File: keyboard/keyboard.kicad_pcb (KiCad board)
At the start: 2 copper layers, 127.1 x 77.5 mm, 21 parts

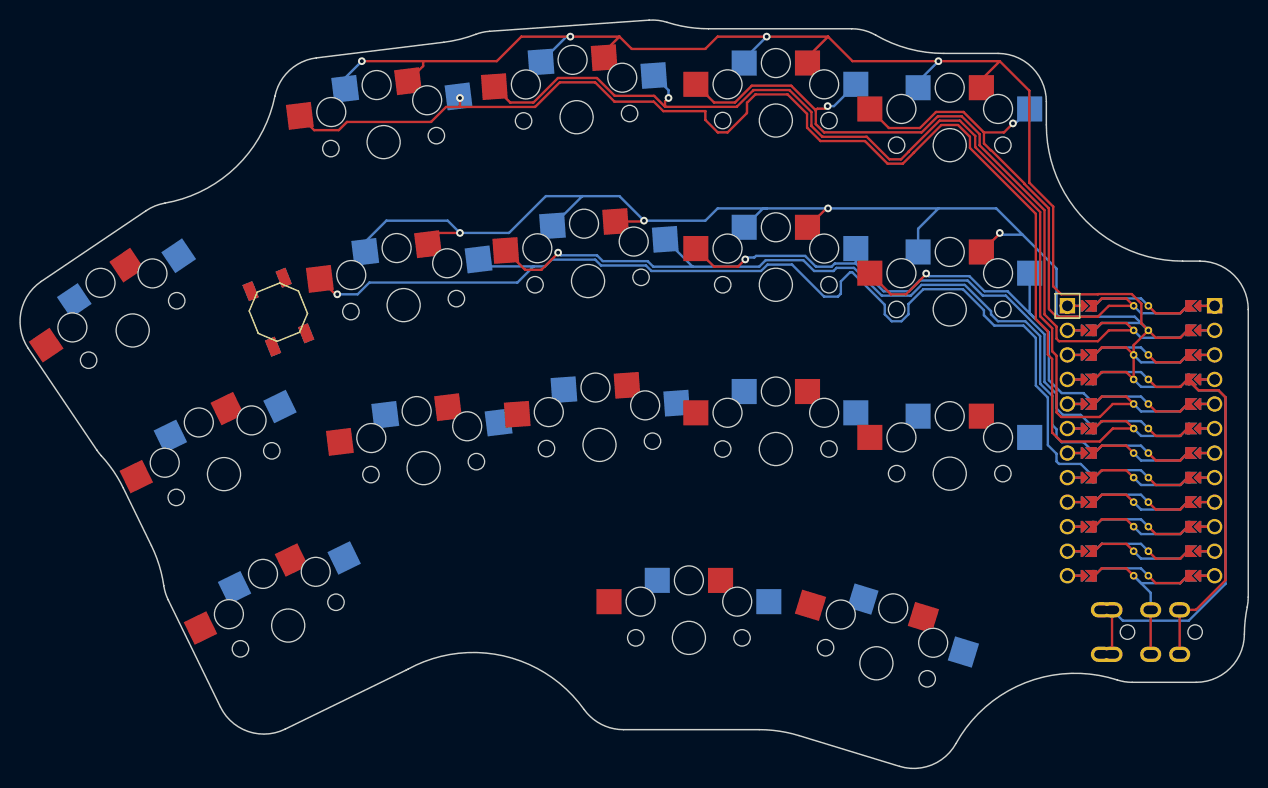
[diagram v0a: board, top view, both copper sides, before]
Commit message: Connect the rest of the stuff
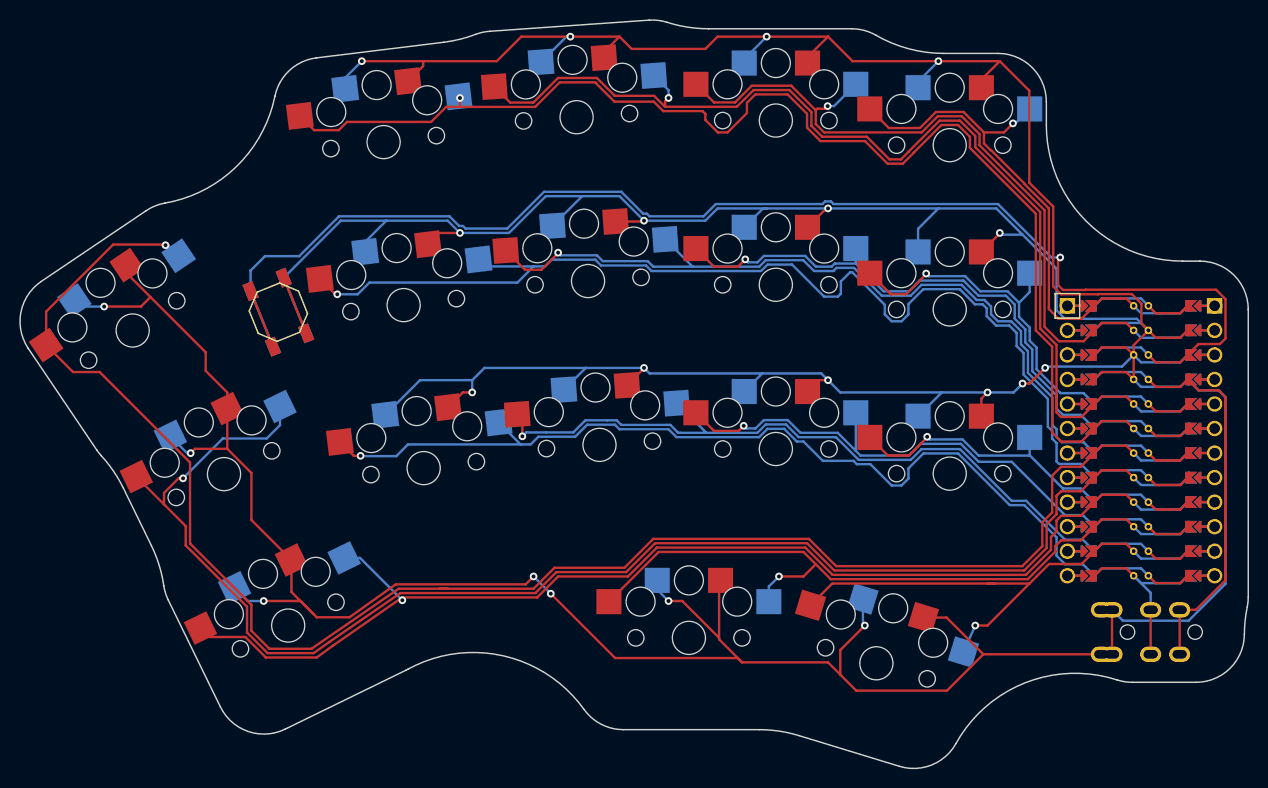
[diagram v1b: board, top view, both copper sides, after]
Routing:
- net GND: track 300.8 -> 623.8 mm, vias 8 -> 21
- net main_pinkie_top: track 0.00 -> 163.2 mm, vias 0 -> 1
- net main_pinkie_home: track 0.00 -> 139.3 mm, vias 0 -> 1
- net RST: track 0.00 -> 136.5 mm, vias 0 -> 1
- net main_pinkie_bottom: track 0.00 -> 111.8 mm, vias 0 -> 1
- net main_ring_bottom: track 0.00 -> 95.0 mm, vias 0 -> 1
- net main_middle_bottom: track 0.00 -> 74.0 mm, vias 0 -> 1
- net thumb_tucky: track 0.00 -> 63.5 mm, vias 0 -> 1
- net main_index_bottom: track 0.00 -> 52.2 mm, vias 0 -> 1
- net thumb_resty: track 0.00 -> 42.9 mm, vias 0 -> 1
- net main_far_bottom: track 0.00 -> 29.5 mm, vias 0 -> 1
- net main_ring_top: track 127.4 -> 123.1 mm
- net main_middle_top: track 104.5 -> 100.4 mm
- net main_index_top: track 73.4 -> 69.4 mm
- net main_far_top: track 50.6 -> 46.7 mm
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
